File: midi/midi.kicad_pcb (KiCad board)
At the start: 2 copper layers, 100 x 96 mm, 11 parts, among them J1 Conn_01x07_Pin, SW1 SW_Push, SW2 SW_Push, SW3 SW_Push, SW4 RotaryEncoder_Switch_MP, U1 Waveshare ESP32-S3-ZERO

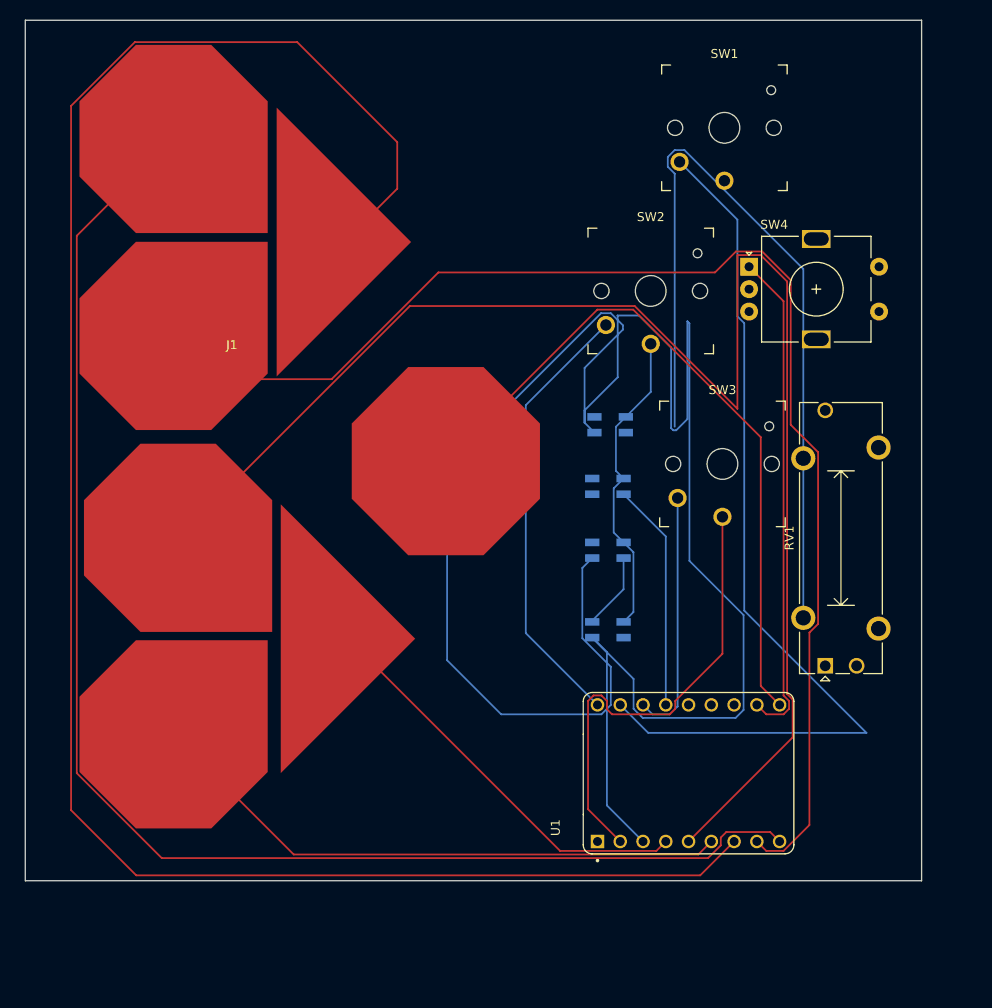
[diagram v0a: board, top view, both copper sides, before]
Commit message: added stuff
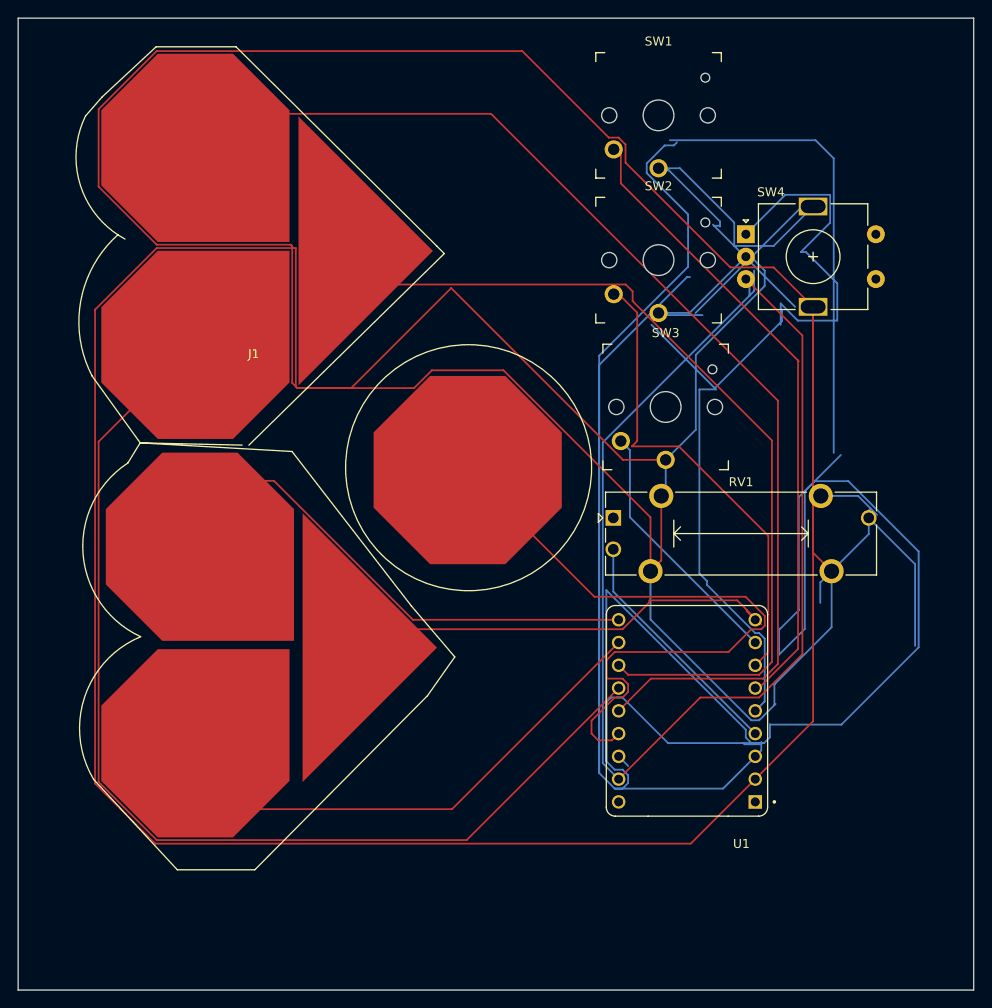
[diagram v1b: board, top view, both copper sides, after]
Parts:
- removed D1, D2, D3, D4: SK6812MINI, LED_SMD:LED_SK6812MINI_PLCC4_3.5x3.5mm_P1.75mm
- added G***: LOGO, LOGO, B.Cu at (82.4, 121.9)
- moved RV1 28.8 mm to (122.6, 128.5), turned to 0 degrees
- moved SW3 8.97 mm to (128.4, 116.1)
- moved SW1 7.48 mm to (127.7, 83.6)
- moved U1 6.96 mm to (130.8, 150.0), turned to 180 degrees
- moved SW4 3.64 mm to (137.4, 96.9)
- moved SW2 3.55 mm to (127.7, 99.8)
- moved J1 2.63 mm to (82.5, 110.7)
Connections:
- U1 pad 1: /TOUCH1 -> /SLIDE
- U1 pad 10: /ENC1_SW -> /TOUCH5
- U1 pad 11: /SLIDE -> /TOUCH6
- U1 pad 12: /LED -> /TOUCH7
- U1 pad 13: /SWITCH3 -> unconnected-(U1-GP13-Pad13)
- U1 pad 2: /TOUCH2 -> /ENC1_A
- U1 pad 3: /TOUCH3 -> /SWITCH1
- U1 pad 4: /TOUCH4 -> /SWITCH2
- U1 pad 5: /TOUCH5 -> /SWITCH3
- U1 pad 6: /TOUCH6 -> /TOUCH1
- U1 pad 7: /TOUCH7 -> /TOUCH2
- U1 pad 8: /ENC1_A -> /TOUCH3
- U1 pad 9: /ENC1_B -> /TOUCH4
- U1 pad RX: /SWITCH1 -> /ENC1_B
- U1 pad TX: /SWITCH2 -> /ENC1_SW
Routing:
- net GND: track 177.5 -> 713.1 mm
- net /ENC1_B: track 0.00 -> 137.0 mm
- net /TOUCH4: track 214.7 -> 97.6 mm
- net /TOUCH2: track 169.3 -> 56.2 mm
- net /ENC1_A: track 55.5 -> 153.7 mm
- net +3V3: track 239.6 -> 331.8 mm
- net /SWITCH1: track 101.1 -> 70.4 mm
- net /TOUCH6: track 159.7 -> 129.1 mm
- net /SLIDE: track 0.00 -> 27.1 mm
- net /TOUCH5: track 148.0 -> 121.0 mm
- net /LED: track 25.5 -> 0.00 mm
- net Net-(D1-VSS): track 8.57 -> 0.00 mm
- net /TOUCH3: track 66.1 -> 58.0 mm
- net /TOUCH1: track 45.7 -> 48.6 mm
- net /SWITCH2: track 49.4 -> 52.1 mm
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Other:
- board size 100 x 96 mm -> 106.6 x 108.4 mm
